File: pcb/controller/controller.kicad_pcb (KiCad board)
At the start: 2 copper layers, 100 x 40 mm, 27 parts, among them J1 Conn_01x02, J10 USB_C_Receptacle_USB2.0_16P, J2 Conn_01x02, J3 Conn_01x02, J4 Conn_01x02, J5 Conn_01x02, J6 Conn_01x02, J7 Conn_01x02, J8 RJ45, U2 AP2112K-3.3

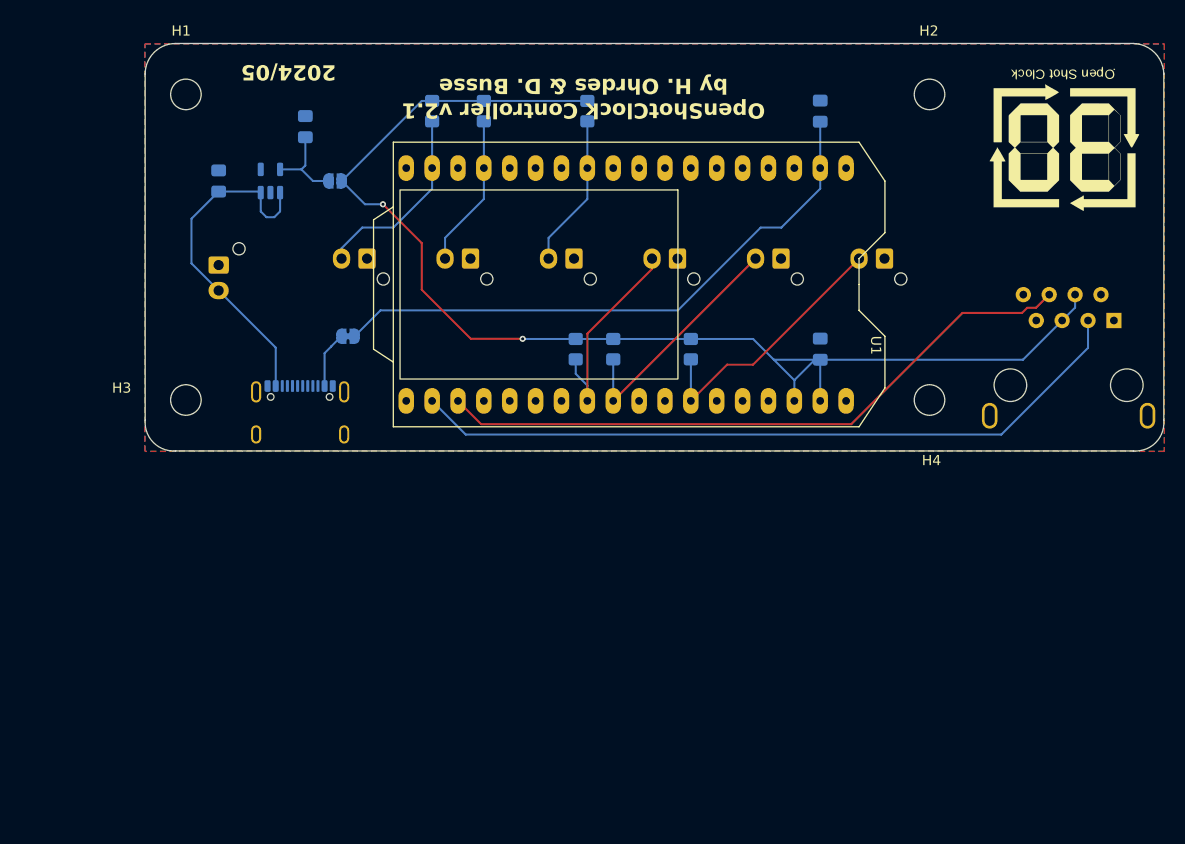
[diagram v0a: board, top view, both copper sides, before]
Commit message: Final Version of new Controller Rev. 00 (Prototype)
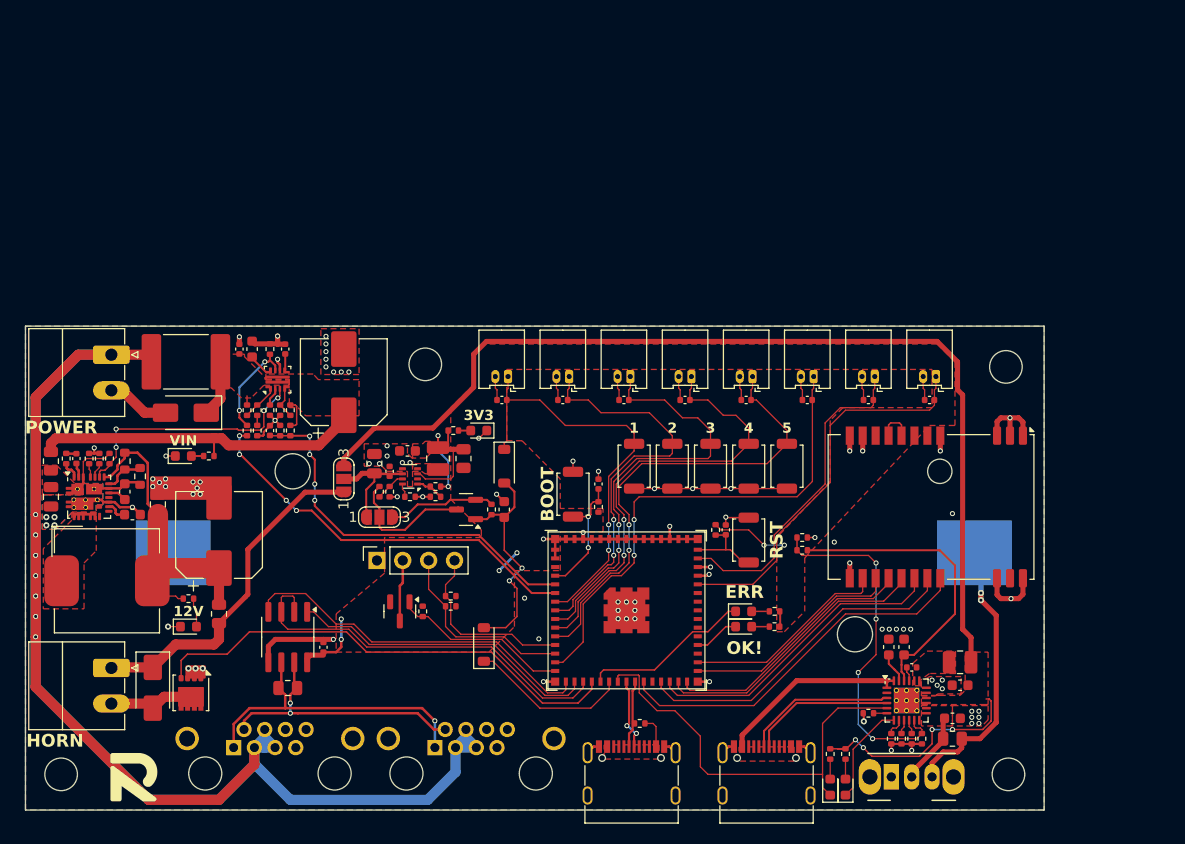
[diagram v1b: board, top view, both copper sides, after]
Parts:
- added BT1: Battery_Cell, Battery:BatteryHolder_Keystone_1042_1x18650, B.Cu at (104.1, 100.0)
- added C10: 100n, Capacitor_SMD:C_0402_1005Metric, F.Cu at (127.0, 85.0)
- added C11: 100n, Capacitor_SMD:C_0402_1005Metric, F.Cu at (79.5, 109.3)
- added C12: 100n, Capacitor_SMD:C_0402_1005Metric, F.Cu at (55.2, 90.7)
- added C13: 1u, Capacitor_SMD:C_0805_2012Metric, F.Cu at (52.8, 94.5)
- added C14: 1u, Capacitor_SMD:C_0603_1608Metric, F.Cu at (60.0, 94.0)
- added C15: 2u2, Capacitor_SMD:C_0603_1608Metric, F.Cu at (60.8, 96.2)
- added C16: 1u, Capacitor_SMD:C_0805_2012Metric, F.Cu at (63.2, 95.2)
- added C17: 100u, Capacitor_SMD:CP_Elec_8x10, F.Cu at (69.2, 98.2)
- added C18: 100n, Capacitor_SMD:C_0402_1005Metric, F.Cu at (71.3, 80.0)
- added C19: 1u, Capacitor_SMD:C_0603_1608Metric, F.Cu at (72.5, 80.0)
- added C20: 1n, Capacitor_SMD:C_0402_1005Metric, F.Cu at (75.8, 80.0)
- added C21: 100u, Capacitor_SMD:CP_Elec_8x10, F.Cu at (81.5, 83.2)
- added C22: 100n, Capacitor_SMD:C_0402_1005Metric, F.Cu at (74.3, 88.0)
- added C23: 100n, Capacitor_SMD:C_0402_1005Metric, F.Cu at (86.0, 92.0)
- added C24: 1u, Capacitor_SMD:C_0805_2012Metric, F.Cu at (84.5, 91.2)
- added C25: 10u, Capacitor_SMD:C_0603_1608Metric, F.Cu at (87.8, 90.0)
- added C26: 100n, Capacitor_SMD:C_0402_1005Metric, F.Cu at (137.2, 111.2)
- added C27: 10u, Capacitor_SMD:C_0603_1608Metric, F.Cu at (142.0, 113.0)
- added C28: 10u, Capacitor_SMD:C_0603_1608Metric, F.Cu at (97.2, 95.8)
- added C29: 10u, Capacitor_SMD:C_0603_1608Metric, F.Cu at (136.5, 109.2)
- added C30: 10u, Capacitor_SMD:C_0603_1608Metric, F.Cu at (141.2, 116.2)
- added C31: 10u, Capacitor_SMD:C_0603_1608Metric, F.Cu at (135.0, 109.2)
- added C5: 100n, Capacitor_SMD:C_0402_1005Metric, F.Cu at (139.0, 85.0)
- added C6: 100n, Capacitor_SMD:C_0402_1005Metric, F.Cu at (133.0, 85.0)
- added C7: 100n, Capacitor_SMD:C_0402_1005Metric, F.Cu at (109.0, 85.0)
- added C8: 100n, Capacitor_SMD:C_0402_1005Metric, F.Cu at (115.0, 85.0)
- added C9: 100n, Capacitor_SMD:C_0402_1005Metric, F.Cu at (121.0, 85.0)
- added D1: LED, LED_SMD:LED_0603_1608Metric, F.Cu at (120.8, 107.2)
- added D10: LED, LED_SMD:LED_0603_1608Metric, F.Cu at (66.3, 107.2)
- added D11: LED, LED_SMD:LED_0603_1608Metric, F.Cu at (94.8, 88.0)
- added D2: LED, LED_SMD:LED_0603_1608Metric, F.Cu at (120.8, 105.8)
- added D3: SMAJ24A, Diode_SMD:D_SMA, F.Cu at (62.8, 113.2)
- added D4: SMAJ24A, Diode_SMD:D_SMA, F.Cu at (66.0, 86.2)
- added D5: LED, LED_SMD:LED_0603_1608Metric, F.Cu at (130.8, 123.0)
- added D6: LED, LED_SMD:LED_0603_1608Metric, F.Cu at (129.2, 123.0)
- added D7: 1N5819, Diode_SMD:D_SOD-123, F.Cu at (97.2, 91.5)
- added D8: 1N5819, Diode_SMD:D_SOD-123, F.Cu at (95.2, 109.0)
- added D9: LED, LED_SMD:LED_0603_1608Metric, F.Cu at (65.8, 90.5)
- added F1: 2.6A, Fuse:Fuse_2920_7451Metric, F.Cu at (66.0, 81.2)
- added G***: LOGO, RVNSPRK_Logo:Ravnsprk_Logo_5mm, F.Cu at (61.0, 122.0)
- added G***: LOGO, RVNSPRK_Markings:JLC-UL_1-2Layer_10mm, B.Cu at (100.2, 87.0)
- added G***: LOGO, Open-Shot-Clock:Open-Shot-Clock_QR_8mm, B.Cu at (56.2, 105.5)
- added G***: LOGO, RVNSPRK_Logo:Ravnsprk_Logo_Mask_5mm, B.Cu at (146.5, 88.8)
- added J11: JST XH, Connector_Molex:Molex_PicoBlade_53048-0210_1x02_P1.25mm_Horizontal, F.Cu at (115.6, 82.7)
- added J12: JST XH, Connector_Molex:Molex_PicoBlade_53048-0210_1x02_P1.25mm_Horizontal, F.Cu at (121.6, 82.7)
- added J13: JST XH, Connector_Molex:Molex_PicoBlade_53048-0210_1x02_P1.25mm_Horizontal, F.Cu at (127.6, 82.7)
- added J9: JST XH, Connector_Molex:Molex_PicoBlade_53048-0210_1x02_P1.25mm_Horizontal, F.Cu at (133.6, 82.7)
- added L1: 10uH, Inductor_SMD:L_Bourns_SRP1050WA, F.Cu at (58.3, 102.7)
- added L2: 2.2uH, Inductor_SMD:L_1008_2520Metric, F.Cu at (90.8, 90.8)
- added L3: 2.2uH, Inductor_SMD:L_1008_2520Metric, F.Cu at (142.0, 110.8)
- added P1: USB_C_Plug_USB2.0, Connector_USB:USB_C_Receptacle_G-Switch_GT-USB-7010ASV, F.Cu at (109.8, 122.8)
- added P2: USB_C_Plug_USB2.0, Connector_USB:USB_C_Receptacle_G-Switch_GT-USB-7010ASV, F.Cu at (123.0, 122.8)
- added Q1: 20N06, Package_SON:VSON-8_3.3x3.3mm_P0.65mm_NexFET, F.Cu at (66.5, 113.8)
- added Q2: SI2301, Package_TO_SOT_SMD:SOT-23, F.Cu at (87.0, 105.8)
- added Q3: SI2301, Package_TO_SOT_SMD:SOT-23, F.Cu at (93.5, 95.8)
- added R10: 0R, Resistor_SMD:R_0805_2012Metric, F.Cu at (52.8, 91.0)
- added R11: 10k, Resistor_SMD:R_0402_1005Metric, F.Cu at (58.5, 90.7)
- added R12: 2R2, Resistor_SMD:R_0402_1005Metric, F.Cu at (54.2, 90.7)
- added R13: 0R, Resistor_SMD:R_0805_2012Metric, F.Cu at (69.2, 106.0)
- added R14: 10k, Resistor_SMD:R_0402_1005Metric, F.Cu at (72.0, 86.0)
- added R15: 10k, Resistor_SMD:R_0402_1005Metric, F.Cu at (76.3, 86.0)
- added R16: 10k, Resistor_SMD:R_0402_1005Metric, F.Cu at (76.3, 88.0)
- added R17: 1k, Resistor_SMD:R_0402_1005Metric, F.Cu at (72.0, 88.0)
- added R18: 82k, Resistor_SMD:R_0603_1608Metric, F.Cu at (60.0, 91.0)
- added R19: 1k, Resistor_SMD:R_0402_1005Metric, F.Cu at (73.0, 86.0)
- added R20: 200k, Resistor_SMD:R_0402_1005Metric, F.Cu at (57.5, 90.7)
- added R21: 200k, Resistor_SMD:R_0402_1005Metric, F.Cu at (56.5, 90.8)
- added R22: 4k3, Resistor_SMD:R_0603_1608Metric, F.Cu at (61.5, 92.5)
- added R23: 560R, Resistor_SMD:R_0402_1005Metric, F.Cu at (73.0, 88.0)
- added R24: 0R, Resistor_SMD:R_0402_1005Metric, F.Cu at (74.3, 86.0)
- added R25: 560R, Resistor_SMD:R_0402_1005Metric, F.Cu at (74.3, 80.0)
- added R26: 1k, Resistor_SMD:R_0402_1005Metric, F.Cu at (75.3, 86.0)
- added R27: 1k, Resistor_SMD:R_0402_1005Metric, F.Cu at (75.3, 88.0)
- added R28: 0R, Resistor_SMD:R_0805_2012Metric, F.Cu at (93.2, 90.8)
- added R29: 1k, Resistor_SMD:R_0402_1005Metric, F.Cu at (130.8, 119.8)
- added R30: 1k, Resistor_SMD:R_0402_1005Metric, F.Cu at (129.2, 119.8)
- added R31: 22k, Resistor_SMD:R_0402_1005Metric, F.Cu at (85.0, 94.0)
- added R32: 200k, Resistor_SMD:R_0402_1005Metric, F.Cu at (90.5, 93.5)
- added R33: 10k, Resistor_SMD:R_0402_1005Metric, F.Cu at (86.0, 94.0)
- added R34: 0R, Resistor_SMD:R_0402_1005Metric, F.Cu at (88.0, 94.5)
- added R35: 47k, Resistor_SMD:R_0402_1005Metric, F.Cu at (90.5, 94.5)
- added R36: 200k, Resistor_SMD:R_0402_1005Metric, F.Cu at (96.0, 95.8)
- added R37: 0R, Resistor_SMD:R_0805_2012Metric, F.Cu at (141.2, 118.2)
- added R38: 10k, Resistor_SMD:R_0402_1005Metric, F.Cu at (126.5, 99.8)
- added R39: 22k, Resistor_SMD:R_0402_1005Metric, F.Cu at (68.2, 90.5)
- added R40: 10k, Resistor_SMD:R_0402_1005Metric, F.Cu at (66.2, 104.5)
- added R41: 1k, Resistor_SMD:R_0402_1005Metric, F.Cu at (92.2, 88.0)
- added R42: 22k, Resistor_SMD:R_0402_1005Metric, F.Cu at (138.2, 118.3)
- added R43: 1k, Resistor_SMD:R_0402_1005Metric, F.Cu at (133.0, 115.8)
- added R44: 1k, Resistor_SMD:R_0402_1005Metric, F.Cu at (136.2, 118.3)
- added R45: 470R, Resistor_SMD:R_0402_1005Metric, F.Cu at (135.2, 118.2)
- added R46: 470R, Resistor_SMD:R_0402_1005Metric, F.Cu at (137.2, 118.3)
- added R7: 1k, Resistor_SMD:R_0402_1005Metric, F.Cu at (106.5, 95.5)
- added R8: 200k, Resistor_SMD:R_0402_1005Metric, F.Cu at (89.2, 105.8)
- added R9: 120R, Resistor_SMD:R_0805_2012Metric, F.Cu at (76.0, 113.3)
- added REF**: OpenShotClock, RVNSPRK_Logo:OpenShotClock, B.Cu at (57.0, 89.5)
- added REF**: OSHW-Logo2_9.8x8mm_SilkScreen, Symbol:OSHW-Logo2_9.8x8mm_SilkScreen, B.Cu at (132.0, 114.8)
- added REF**: KiCad-Logo2_6mm_SilkScreen, Symbol:KiCad-Logo2_6mm_SilkScreen, B.Cu at (119.3, 113.8)
- added SW1: SW_4x3mm, RVNSPRK_Switch:SW_Push_4x3mm, F.Cu at (121.2, 98.8)
- added SW2: SW_4x3mm, RVNSPRK_Switch:SW_Push_4x3mm, F.Cu at (104.0, 94.2)
- added SW3: SW_4x3mm, RVNSPRK_Switch:SW_Push_4x3mm, F.Cu at (110.0, 91.5)
- added SW4: SW_4x3mm, RVNSPRK_Switch:SW_Push_4x3mm, F.Cu at (113.8, 91.5)
- added SW5: SW_4x3mm, RVNSPRK_Switch:SW_Push_4x3mm, F.Cu at (117.5, 91.5)
- added SW6: SW_4x3mm, RVNSPRK_Switch:SW_Push_4x3mm, F.Cu at (121.2, 91.5)
- added SW7: SW_4x3mm, RVNSPRK_Switch:SW_Push_4x3mm, F.Cu at (125.0, 91.5)
- added SW8: SW_SPDT_312, Button_Switch_THT:SW_CuK_OS102011MA1QN1_SPDT_Angled, F.Cu at (135.3, 122.0)
- added TH1: NTC, Resistor_SMD:R_0402_1005Metric, F.Cu at (126.5, 98.5)
- added U*1: BQ25606, Package_DFN_QFN:VQFN-24-1EP_4x4mm_P0.5mm_EP2.5x2.5mm_ThermalVias, F.Cu at (136.8, 114.5)
- added U3: E220-400M22S, RVNSPRK_Modules:E220-400M22S, F.Cu at (139.2, 95.5)
- added U4: SIC438BED-T1-GE3, Package_DFN_QFN:Vishay_PowerPAK_MLP44-24L_ThermalVias, F.Cu at (56.5, 94.5)
- added U5: TPS259474x, RVNSPRK_Packages:RPW0010A_VQFN-HR-10, F.Cu at (75.0, 83.0)
- added U6: TPS629206, Package_TO_SOT_SMD:SOT-583-8, F.Cu at (88.0, 92.5)
- C1, C2, C3, C4: value C -> 100n; footprint Capacitor_SMD:C_0805_2012Metric_Pad1.18x1.45mm_HandSolder -> Capacitor_SMD:C_0402_1005Metric; moved to F.Cu
- H1, H2, H3, H4: value MountingHole -> M3; footprint MountingHole:MountingHole_3mm -> MountingHole:MountingHole_3.2mm_M3
- J1, J4: value Conn_01x02 -> Term 3.5mm; footprint Connector_JST:JST_XH_B2B-XH-AM_1x02_P2.50mm_Vertical -> Connector_Phoenix_MC:PhoenixContact_MC_1,5_2-G-3.5_1x02_P3.50mm_Horizontal; moved to F.Cu
- J10: value USB_C_Receptacle_USB2.0_16P -> JST XH; footprint Connector_USB:USB_C_Receptacle_GCT_USB4105-xx-A_16P_TopMnt_Horizontal -> Connector_Molex:Molex_PicoBlade_53048-0210_1x02_P1.25mm_Horizontal; moved to F.Cu
- J2, J3: value Conn_01x02 -> RJ45; footprint Connector_JST:JST_XH_B2B-XH-AM_1x02_P2.50mm_Vertical -> Connector_RJ:RJ45_Amphenol_RJHSE5380
- J5: value Conn_01x02 -> OLED 0.96" (I2C); footprint Connector_JST:JST_XH_B2B-XH-AM_1x02_P2.50mm_Vertical -> Connector_PinSocket_2.54mm:PinSocket_1x04_P2.54mm_Vertical; moved to F.Cu
- J6, J7: value Conn_01x02 -> JST XH; footprint Connector_JST:JST_XH_B2B-XH-AM_1x02_P2.50mm_Vertical -> Connector_Molex:Molex_PicoBlade_53048-0210_1x02_P1.25mm_Horizontal; moved to F.Cu
- J8: value RJ45 -> JST XH; footprint RJ45:RJ45_Amphenol_54602-x08_Horizontal -> Connector_Molex:Molex_PicoBlade_53048-0210_1x02_P1.25mm_Horizontal; moved to F.Cu
- JP1: value SolderJumper_2_Bridged -> SolderJumper_3_Open; footprint Jumper:SolderJumper-2_P1.3mm_Bridged_RoundedPad1.0x1.5mm -> Jumper:SolderJumper-3_P1.3mm_Open_RoundedPad1.0x1.5mm_NumberLabels; moved to F.Cu
- JP2: value SolderJumper_2_Open -> SolderJumper_3_Open; footprint Jumper:SolderJumper-2_P1.3mm_Open_RoundedPad1.0x1.5mm -> Jumper:SolderJumper-3_P1.3mm_Open_RoundedPad1.0x1.5mm_NumberLabels; moved to F.Cu
- R1, R2, R3, R4: value 10k -> 1k; footprint Resistor_SMD:R_0805_2012Metric_Pad1.20x1.40mm_HandSolder -> Resistor_SMD:R_0402_1005Metric; moved to F.Cu
- R5, R6: value 10k -> 4k3; footprint Resistor_SMD:R_0805_2012Metric_Pad1.20x1.40mm_HandSolder -> Resistor_SMD:R_0402_1005Metric; moved to F.Cu
- U1: value ~ -> ESP32-S3-MINI-1; footprint Heltec_WiFi_LoRa_V3:Heltec_WiFi_LoRa_V3 -> Espressif:ESP32-S3-MINI-1U
- U2: value AP2112K-3.3 -> SP3485EN; footprint Package_TO_SOT_SMD:SOT-23-5 -> Package_SO:SOIC-8_3.9x4.9mm_P1.27mm; moved to F.Cu
- moved H4 92.8 mm to (53.8, 121.8), turned to 90 degrees
- moved H3 88.7 mm to (146.8, 121.8), turned to 90 degrees
- moved J1 76.5 mm to (58.7, 80.6), turned to -90 degrees
- moved J3 64.8 mm to (70.7, 119.1), turned to 0 degrees
- moved R3 63.5 mm to (110.5, 116.8), turned to 180 degrees
- moved J4 60.6 mm to (58.7, 111.3), turned to -90 degrees
- moved J2 58.8 mm to (90.4, 119.1), turned to 0 degrees
- moved C1 57.2 mm to (119.0, 97.8), turned to 90 degrees
- moved R2 56.8 mm to (123.8, 105.8), turned to 180 degrees
- moved R1 53.8 mm to (123.8, 107.2), turned to 180 degrees
- moved C2 47.7 mm to (106.5, 93.2), turned to 90 degrees
- moved U2 44.8 mm to (76.0, 108.3), turned to -90 degrees
- moved C3 42.2 mm to (97.0, 85.0), turned to 180 degrees
- moved J7 36.1 mm to (103.6, 82.7), turned to 180 degrees
- moved H1 35.4 mm to (89.5, 81.5), turned to 90 degrees
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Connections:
- C1 pad 1: GND -> Net-(U1-EN)
- C1 pad 2: Net-(JP2-B) -> GND
- C2 pad 1: GND -> /BOOT
- C2 pad 2: 5V_IN -> GND
- C3 pad 1: 5V -> /BTN_1
- C4 pad 1: 3V3 -> /BTN_2
- J1 pad 1: GND -> VBUS
- J1 pad 2: GPIO42 -> GND
- J2 pad 1: GND -> /Communication/RS485.A
- J2 pad 2: GPIO39 -> /Communication/RS485.B
- J3 pad 1: GND -> /Communication/RS485.A
- J3 pad 2: GPIO38 -> /Communication/RS485.B
- J4 pad 1: GND -> +12V
- J4 pad 2: GPIO34 -> Net-(D3-A2)
- J5 pad 2: GPIO26 -> Net-(J5-Pin_2)
- J6 pad 1: GND -> /BTN_1
- J6 pad 2: GPIO20 -> GND
- J7 pad 1: GND -> /BTN_2
- J7 pad 2: 5V_IN -> GND
- J8 pad 1: unconnected-(J8-Pad1) -> /BTN_8
- J8 pad 2: unconnected-(J8-Pad2) -> GND
- JP1 pad 1: 5V -> +12V
- JP1 pad 2: 5V_IN -> Net-(JP1-C)
- JP2 pad 1: 3V3 -> Net-(JP1-C)
- JP2 pad 2: Net-(JP2-B) -> Net-(JP2-C)
- R1 pad 1: GPIO34 -> +3.3V
- R1 pad 2: 3V3 -> Net-(D1-A)
- R2 pad 1: GPIO26 -> +3.3V
- R2 pad 2: 3V3 -> Net-(D2-A)
- R3 pad 1: GPIO20 -> /VUSB
- R3 pad 2: 3V3 -> /D_P
- R4 pad 1: GPIO42 -> +3.3V
- R4 pad 2: 3V3 -> Net-(U1-EN)
- R5 pad 1: GPIO39 -> +3.3V
- R5 pad 2: 3V3 -> /I2C.SDA
- R6 pad 1: GPIO38 -> +3.3V
- R6 pad 2: 3V3 -> /I2C.SCL
- U1 pad 10: unconnected-(U1-GPIO35-Pad10) -> /BTN_4
- U1 pad 11: GPIO34 -> /BTN_5
- U1 pad 12: unconnected-(U1-GPIO33-Pad12) -> /I2C.SDA
- U1 pad 13: unconnected-(U1-GPIO47-Pad13) -> /I2C.SCL
- U1 pad 14: unconnected-(U1-GPIO48-Pad14) -> /BTN_6
- U1 pad 15: GPIO26 -> /OLED_EN
- U1 pad 16: unconnected-(U1-GPIO21-Pad16) -> /UART.TX
- U1 pad 17: GPIO20 -> /UART.RX
- U1 pad 18: unconnected-(U1-GPIO19-Pad18) -> /UART.TXEN
- U1 pad 19: GND -> /HORN
- U1 pad 2: 5V -> GND
- U1 pad 20: 3V3 -> /LED.ERR
- U1 pad 21: 3V3 -> /PWR_SHDN
- U1 pad 22: unconnected-(U1-GPIO37-Pad22) -> /CHG_STAT
- U1 pad 23: unconnected-(U1-GPIO46-Pad23) -> /D_N
- U1 pad 24: unconnected-(U1-GPIO45-Pad24) -> /D_P
- U1 pad 25: GPIO42 -> /LORA.NSS
- U1 pad 27: unconnected-(U1-GPIO40-Pad27) -> /SPI.CLK
- U1 pad 28: GPIO39 -> /SPI.MOSI
- U1 pad 29: GPIO38 -> /SPI.MISO
- U1 pad 3: unconnected-(U1-Ve-Pad3) -> +3.3V
- U1 pad 30: unconnected-(U1-GPIO1-Pad30) -> /LORA.RST
- U1 pad 31: unconnected-(U1-GPIO2-Pad31) -> /LORA.BUSY
- U1 pad 32: unconnected-(U1-GPIO3-Pad32) -> /LORA.IRQ
- U1 pad 34: TX2 -> /LED.OK
- U1 pad 35: RX2 -> unconnected-(U1-MTCK/GPIO39/CLK_OUT3/SUBSPICS1-Pad35)
- U1 pad 4: unconnected-(U1-Ve-Pad4) -> /BOOT
- U1 pad 5: unconnected-(U1-RX-Pad5) -> /V_SENSE
- U1 pad 6: unconnected-(U1-TX-Pad6) -> /I_SENSE
- U1 pad 7: unconnected-(U1-RST-Pad7) -> /BTN_1
- U1 pad 8: unconnected-(U1-GPIO0-Pad8) -> /BTN_2
- U1 pad 9: unconnected-(U1-GPIO36-Pad9) -> /BTN_3
- U2 pad 1: 5V_IN -> /UART.RX
- U2 pad 2: GND -> /UART.TXEN
- U2 pad 3: 5V_IN -> /UART.TXEN
- U2 pad 4: unconnected-(U2-NC-Pad4) -> /UART.TX
- U2 pad 5: Net-(JP2-B) -> GND
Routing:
- net VBUS: track 0.00 -> 173.8 mm, vias 0 -> 7
- net GND: track 0.00 -> 144.8 mm, vias 0 -> 94
- net 3V3: track 125.0 -> 0.00 mm, vias 2 -> 0
- net VSYS: track 0.00 -> 120.9 mm, vias 0 -> 4
- net RX2: track 72.8 -> 0.00 mm
- net TX2: track 64.3 -> 0.00 mm
- net 5V: track 58.3 -> 0.00 mm
- net /BTN_6: track 0.00 -> 48.7 mm, vias 0 -> 2
- net /HORN: track 0.00 -> 47.4 mm
- net /BTN_5: track 0.00 -> 46.3 mm, vias 0 -> 2
- net /BTN_4: track 0.00 -> 43.7 mm, vias 0 -> 2
- net /BTN_3: track 0.00 -> 42.0 mm, vias 0 -> 2
- net /CHG_STAT: track 0.00 -> 41.8 mm
- net /BTN_1: track 0.00 -> 41.6 mm, vias 0 -> 2
- net /BTN_2: track 0.00 -> 39.5 mm, vias 0 -> 2
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- added copper zone on F.Cu, net +3.3V
- added copper zone on F.Cu, net +BATT
- added copper zone on F.Cu, net /Power Supply/3V3_T
- added copper zone on F.Cu, net /VUSB
- added copper zone on F.Cu, net Net-(C26-Pad1)
- added copper zone on F.Cu, net Net-(D4-A1)
- added copper zone on F.Cu, net Net-(U*1-VAC)
- added copper zone on F.Cu, net Net-(U6-SW)
- added copper zone on F.Cu, net SW
- added copper zone on F.Cu, net VCC
- added copper zone on F.Cu, net VIN
- added copper zone on F.Cu, net VSYS
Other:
- board size 100 x 40 mm -> 100 x 47.5 mm
- board text added: "1"
- board text added: "12V"
- board text added: "2"
- board text added: "3"
- board text added: "3V3"
- board text added: "4"
- board text added: "5"
- board text added: "BOOT"
- board text added: "ERR"
- board text added: "GitHub"
- board text added: "HORN"
- board text added: "OK!"
- board text added: "Open Shot Clock Controller"
- board text added: "POWER"
- board text added: "RST"
- board text added: "Rev. 00 яαvεηsραяκ 2024"
- board text added: "VIN"
- board text removed: "+"
- board text removed: "-"
- board text removed: "2024/05"
- board text removed: "5V"
- board text removed: "GND"
- board text removed: "OpenShotClock Controller v2.1"
- board text removed: "OpenShotClock Controller v2.1 by H. Ohrdes & D. Busse"
